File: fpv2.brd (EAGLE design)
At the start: 100 x 100 mm, 78 parts, among them J1 MOT1, J101 SWD, J11 5V, J12 5V, J13 5V, J2 MOT2, J21 USB, J3 MOT3, J4 MOT4, J5 S.BUS, Q1 IRLR7843, Q2 IRLR7843, Q3 IRLR7843, Q4 IRLR7843, Q5 MMBT3904, U1 STM32F407VGT6, U4 MIC5219 3.3V, Y1 8M

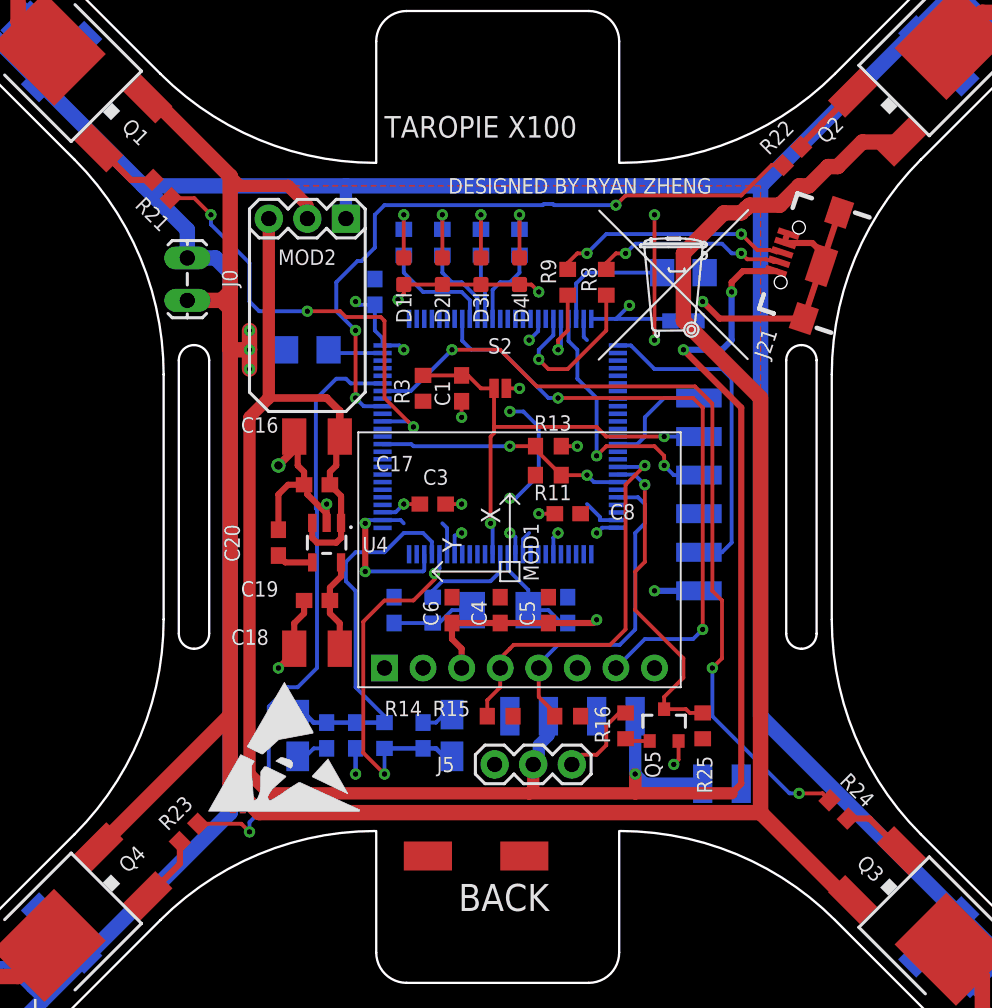
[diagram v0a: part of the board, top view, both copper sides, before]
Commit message: Add files via upload
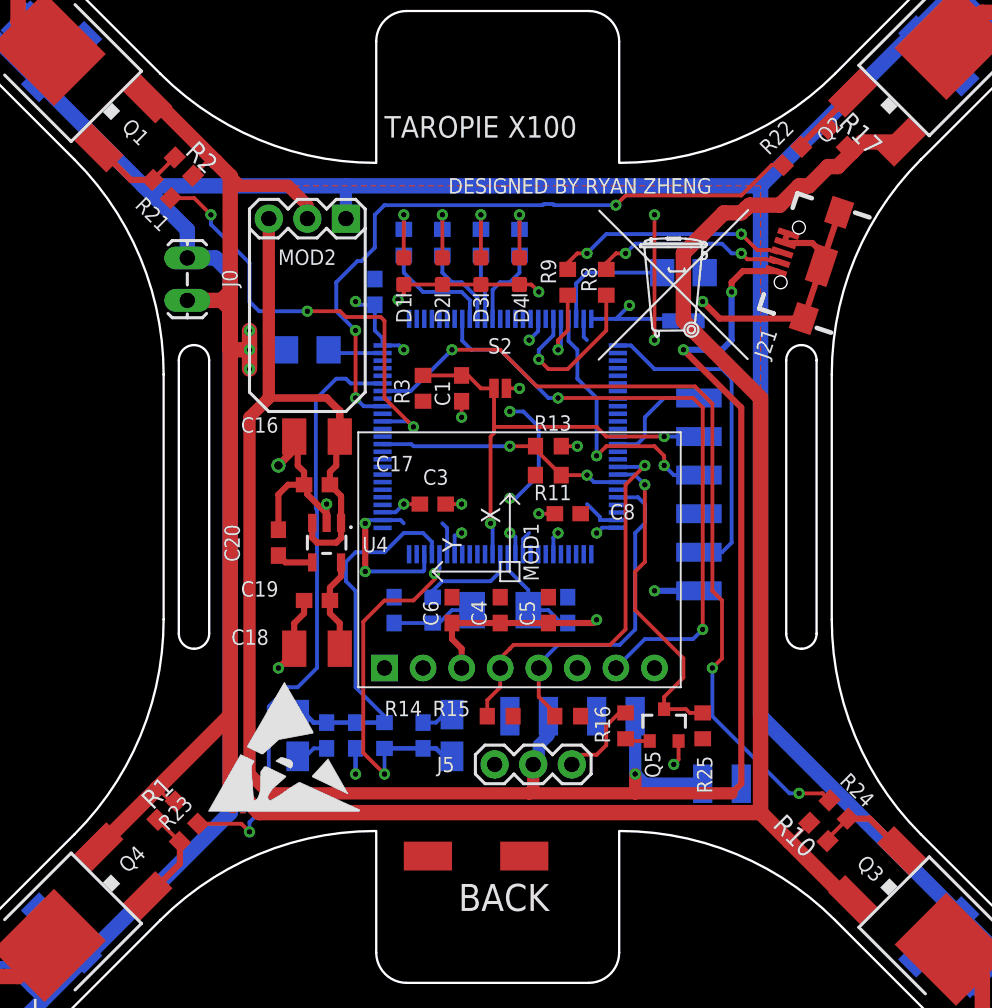
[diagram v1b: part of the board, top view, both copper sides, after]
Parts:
- added R1, R10, R17, R2: 10k, rcl:R0603
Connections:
- net AGND: now also R1.2, R10.2, R17.2, R2.2
- net N$12: now also R2.1
- net N$15: now also R10.1
- net N$17: now also R17.1
- net N$8: now also R1.1
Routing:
- net AGND: track 174.8 -> 180.6 mm
- net N$8: track 4.42 -> 6.50 mm
- net N$12: track 4.42 -> 6.50 mm
- net N$15: track 4.42 -> 6.45 mm
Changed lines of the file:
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@@
 <grid distance="25" unitdist="mil" unit="mil" style="lines" multiple="1" display="yes" altdistance="5" altunitdist="mil" altunit="mil"/>
 <layers>
-<layer number="1" name="Top" color="4" fill="1" visible="yes" active="yes"/>
+<layer number="1" name="Top" color="4" fill="1" visible="no" active="yes"/>
 <layer number="2" name="Route2" color="1" fill="3" visible="no" active="no"/>
 <layer number="3" name="Route3" color="4" fill="3" visible="no" active="no"/>
@@
 <layer number="19" name="Unrouted" color="6" fill="1" visible="yes" active="yes"/>
 <layer number="20" name="Dimension" color="15" fill="1" visible="yes" active="yes"/>
-<layer number="21" name="tPlace" color="7" fill="1" visible="yes" active="yes"/>
+<layer number="21" name="tPlace" color="7" fill="1" visible="no" active="yes"/>
 <layer number="22" name="bPlace" color="7" fill="1" visible="yes" active="yes"/>
-<layer number="23" name="tOrigins" color="15" fill="1" visible="yes" active="yes"/>
+<layer number="23" name="tOrigins" color="15" fill="1" visible="no" active="yes"/>
 <layer number="24" name="bOrigins" color="15" fill="1" visible="yes" active="yes"/>
-<layer number="25" name="tNames" color="7" fill="1" visible="yes" active="yes"/>
+<layer number="25" name="tNames" color="7" fill="1" visible="no" active="yes"/>
 <layer number="26" name="bNames" color="7" fill="1" visible="yes" active="yes"/>
-<layer number="27" name="tValues" color="7" fill="1" visible="yes" active="yes"/>
-<layer number="28" name="bValues" color="7" fill="1" visible="yes" active="yes"/>
+<layer number="27" name="tValues" color="7" fill="1" visible="no" active="yes"/>
+<layer number="28" name="bValues" color="7" fill="1" visible="no" active="yes"/>
 <layer number="29" name="tStop" color="7" fill="3" visible="no" active="yes"/>
 <layer number="30" name="bStop" color="7" fill="6" visible="no" active="yes"/>
@@
 <layer number="37" name="tTest" color="7" fill="1" visible="no" active="yes"/>
 <layer number="38" name="bTest" color="7" fill="1" visible="no" active="yes"/>
-<layer number="39" name="tKeepout" color="4" fill="11" visible="yes" active="yes"/>
+<layer number="39" name="tKeepout" color="4" fill="11" visible="no" active="yes"/>
 <layer number="40" name="bKeepout" color="1" fill="11" visible="yes" active="yes"/>
-<layer number="41" name="tRestrict" color="4" fill="10" visible="yes" active="yes"/>
+<layer number="41" name="tRestrict" color="4" fill="10" visible="no" active="yes"/>
 <layer number="42" name="bRestrict" color="1" fill="10" visible="yes" active="yes"/>
 <layer number="43" name="vRestrict" color="2" fill="10" visible="no" active="yes"/>
-<layer number="44" name="Drills" color="7" fill="1" visible="yes" active="yes"/>
+<layer number="44" name="Drills" color="7" fill="1" visible="no" active="yes"/>
 <layer number="45" name="Holes" color="7" fill="1" visible="yes" active="yes"/>
 <layer number="46" name="Milling" color="3" fill="1" visible="no" active="yes"/>
@@
 <layer number="49" name="Reference" color="7" fill="1" visible="no" active="yes"/>
 <layer number="50" name="dxf" color="7" fill="1" visible="no" active="no"/>
-<layer number="51" name="tDocu" color="7" fill="1" visible="yes" active="yes"/>
+<layer number="51" name="tDocu" color="7" fill="1" visible="no" active="yes"/>
 <layer number="52" name="bDocu" color="7" fill="1" visible="yes" active="yes"/>
 <layer number="53" name="tGND_GNDA" color="7" fill="9" visible="no" active="no"/>
@@
 <element name="U$1" library="logo" package="TONNE_10.00" value="" x="61.468" y="61.976"/>
 <element name="U$2" library="logo" package="ESD_10.00" value="" x="30.861" y="29.21"/>
+<element name="R1" library="rcl" package="R0603" value="10k" x="28.194" y="29.337" rot="R45"/>
+<element name="R2" library="rcl" package="R0603" value="10k" x="29.337" y="71.755" rot="R315"/>
+<element name="R10" library="rcl" package="R0603" value="10k" x="71.12" y="27.94" rot="R135"/>
+<element name="R17" library="rcl" package="R0603" value="10k" x="72.39" y="73.66" rot="R315"/>
 </elements>
 <signals>
@@
 <wire x1="29.0711875" y1="27.2751375" x2="29.0711875" y2="25.84678125" width="0.4064" layer="1"/>
 <wire x1="29.0711875" y1="25.84678125" x2="26.9569375" y2="23.73253125" width="0.4064" layer="1"/>
+<contactref element="R1" pad="1"/>
+<wire x1="27.59295625" y1="28.73595625" x2="27.61036875" y2="28.73595625" width="0.254" layer="1"/>
+<wire x1="27.61036875" y1="28.73595625" x2="29.0711875" y2="27.2751375" width="0.254" layer="1"/>
 </signal>
 <signal name="N$12">
@@
 <wire x1="27.2751375" y1="70.8778125" x2="25.846778125" y2="70.8778125" width="0.4064" layer="1"/>
 <wire x1="25.846778125" y1="70.8778125" x2="23.73253125" y2="72.992059375" width="0.4064" layer="1"/>
+<contactref element="R2" pad="1"/>
+<wire x1="28.73595625" y1="72.356040625" x2="27.2751375" y2="70.895221875" width="0.254" layer="1"/>
+<wire x1="27.2751375" y1="70.895221875" x2="27.2751375" y2="70.8778125" width="0.254" layer="1"/>
 </signal>
 <signal name="N$15">
@@
 <wire x1="73.0548625" y1="28.8171875" x2="74.483215625" y2="28.8171875" width="0.4064" layer="1"/>
 <wire x1="74.483215625" y1="28.8171875" x2="76.597465625" y2="26.7029375" width="0.4064" layer="1"/>
+<contactref element="R10" pad="1"/>
+<wire x1="71.721040625" y1="27.33895625" x2="71.721040625" y2="27.483365625" width="0.254" layer="1"/>
+<wire x1="71.721040625" y1="27.483365625" x2="73.0548625" y2="28.8171875" width="0.254" layer="1"/>
 </signal>
 <signal name="N$17">
 <contactref element="Q2" pad="1"/>
 <contactref element="R22" pad="2"/>
-<wire x1="71.412796875" y1="74.637203125" x2="71.2588125" y2="74.48321875" width="0.4064" layer="1"/>
+<wire x1="71.412796875" y1="74.637203125" x2="69.9888125" y2="73.21321875" width="0.4064" layer="1"/>
 <wire x1="71.412796875" y1="74.637203125" x2="73.373059375" y2="76.597465625" width="0.4064" layer="1"/>
 <wire x1="69.9888125" y1="73.0548625" x2="69.9888125" y2="73.21321875" width="0.4064" layer="1"/>
-<wire x1="69.9888125" y1="73.21321875" x2="71.412796875" y2="74.637203125" width="0.4064" layer="1"/>
+<contactref element="R17" pad="1"/>
+<wire x1="71.78895625" y1="74.261040625" x2="71.78895625" y2="74.26104375" width="0.254" layer="1"/>
+<wire x1="71.78895625" y1="74.26104375" x2="71.412796875" y2="74.637203125" width="0.254" layer="1"/>
 </signal>
 <signal name="AGND">
@@
 <wire x1="32.385" y1="71.12" x2="32.385" y2="63.5" width="1.016" layer="1"/>
 <wire x1="32.385" y1="63.5" x2="32.385" y2="35.60940625" width="1.016" layer="1"/>
-<wire x1="32.385" y1="35.60940625" x2="23.73253125" y2="26.9569375" width="1.016" layer="1"/>
+<wire x1="27.597796875" y1="30.822203125" x2="32.385" y2="35.60940625" width="1.016" layer="1"/>
+<wire x1="27.597796875" y1="30.822203125" x2="23.73253125" y2="26.9569375" width="1.016" layer="1"/>
 <wire x1="32.385" y1="35.60940625" x2="32.385" y2="31.115" width="1.016" layer="1"/>
 <wire x1="32.385" y1="31.115" x2="34.29" y2="29.21" width="1.016" layer="1"/>
 <wire x1="67.31" y1="29.21" x2="34.29" y2="29.21" width="1.016" layer="1"/>
-<wire x1="67.31" y1="29.21" x2="73.66" y2="22.86" width="1.016" layer="1"/>
+<wire x1="69.215" y1="27.305" x2="67.31" y2="29.21" width="1.016" layer="1"/>
+<wire x1="69.215" y1="27.305" x2="73.66" y2="22.86" width="1.016" layer="1"/>
 <wire x1="73.66" y1="22.86" x2="73.66" y2="23.191590625" width="1.016" layer="1"/>
 <wire x1="73.66" y1="23.191590625" x2="73.373059375" y2="23.47853125" width="1.016" layer="1"/>
@@
 <wire x1="32.385" y1="62.386" x2="31.828" y2="62.943" width="1.016" layer="1"/>
 <wire x1="26.9569375" y1="76.216465625" x2="27.288534375" y2="76.216465625" width="1.016" layer="1"/>
-<wire x1="27.288534375" y1="76.216465625" x2="32.385" y2="71.12" width="1.016" layer="1"/>
+<wire x1="31.4325" y1="72.0725" x2="27.288534375" y2="76.216465625" width="1.016" layer="1"/>
+<wire x1="31.4325" y1="72.0725" x2="32.385" y2="71.12" width="1.016" layer="1"/>
 <wire x1="76.597465625" y1="73.373059375" x2="74.008059375" y2="73.373059375" width="1.016" layer="1"/>
-<wire x1="74.008059375" y1="73.373059375" x2="72.39" y2="71.755" width="1.016" layer="1"/>
+<wire x1="73.3425" y1="72.7075" x2="74.008059375" y2="73.373059375" width="1.016" layer="1"/>
+<wire x1="73.3425" y1="72.7075" x2="72.39" y2="71.755" width="1.016" layer="1"/>
 <wire x1="72.39" y1="71.755" x2="71.755" y2="71.755" width="1.016" layer="1"/>
 <wire x1="71.755" y1="71.755" x2="70.485" y2="70.485" width="1.016" layer="1"/>
@@
 <wire x1="64.897" y1="68.707" x2="62.23" y2="66.04" width="1.016" layer="1"/>
 <wire x1="62.23" y1="61.595" x2="67.31" y2="56.515" width="1.016" layer="1"/>
+<contactref element="R17" pad="2"/>
+<contactref element="R10" pad="2"/>
+<contactref element="R1" pad="2"/>
+<contactref element="R2" pad="2"/>
+<wire x1="72.991040625" y1="73.05895625" x2="72.99104375" y2="73.05895625" width="0.254" layer="1"/>
+<wire x1="72.99104375" y1="73.05895625" x2="73.3425" y2="72.7075" width="0.254" layer="1"/>
+<wire x1="29.938040625" y1="71.15395625" x2="30.856584375" y2="72.0725" width="0.254" layer="1"/>
+<wire x1="30.856584375" y1="72.0725" x2="31.4325" y2="72.0725" width="0.254" layer="1"/>
+<wire x1="28.795040625" y1="29.938040625" x2="28.481959375" y2="29.938040625" width="0.254" layer="1"/>
+<wire x1="28.481959375" y1="29.938040625" x2="27.597796875" y2="30.822203125" width="0.254" layer="1"/>
+<wire x1="70.51895625" y1="28.541040625" x2="69.282915625" y2="27.305" width="0.254" layer="1"/>
+<wire x1="69.282915625" y1="27.305" x2="69.215" y2="27.305" width="0.254" layer="1"/>
 </signal>
 <signal name="N$21">
